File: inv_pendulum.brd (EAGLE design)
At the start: 55.5 x 77.5 mm, 9 parts

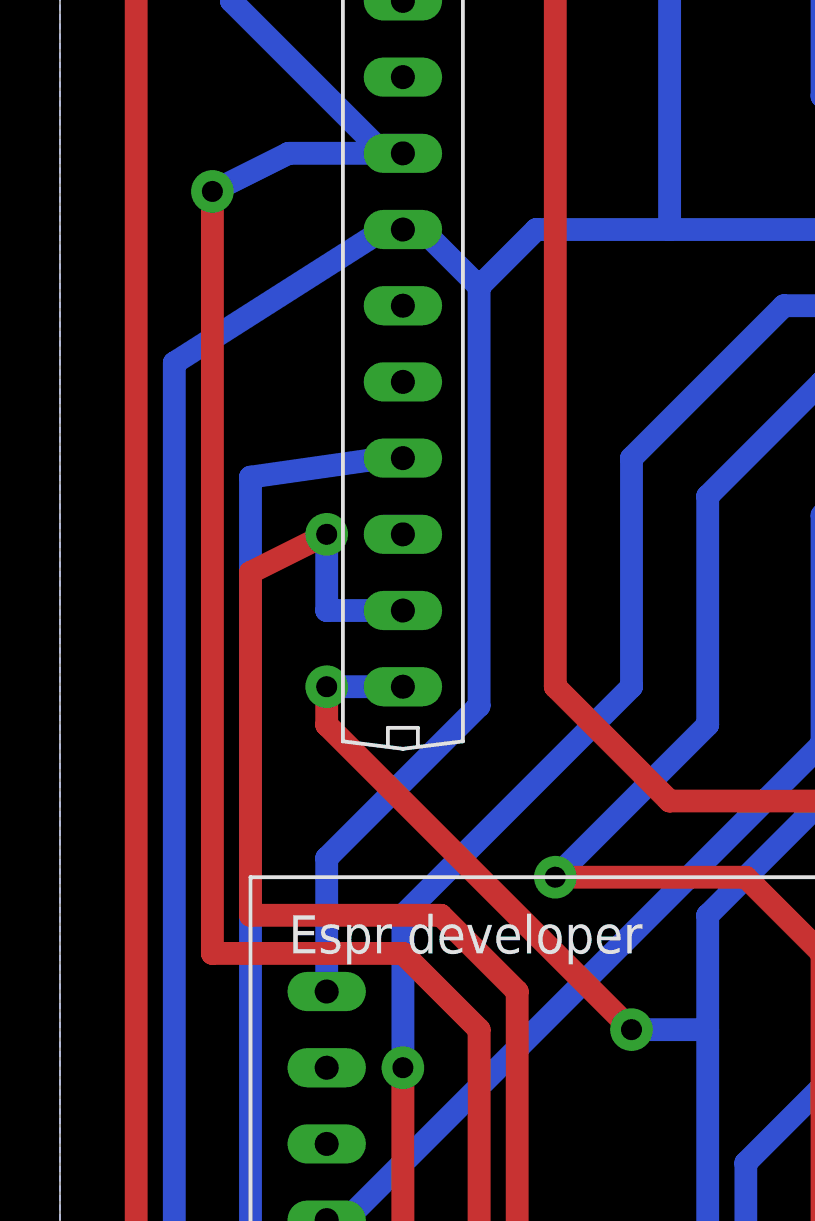
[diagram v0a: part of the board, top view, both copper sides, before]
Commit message: update design
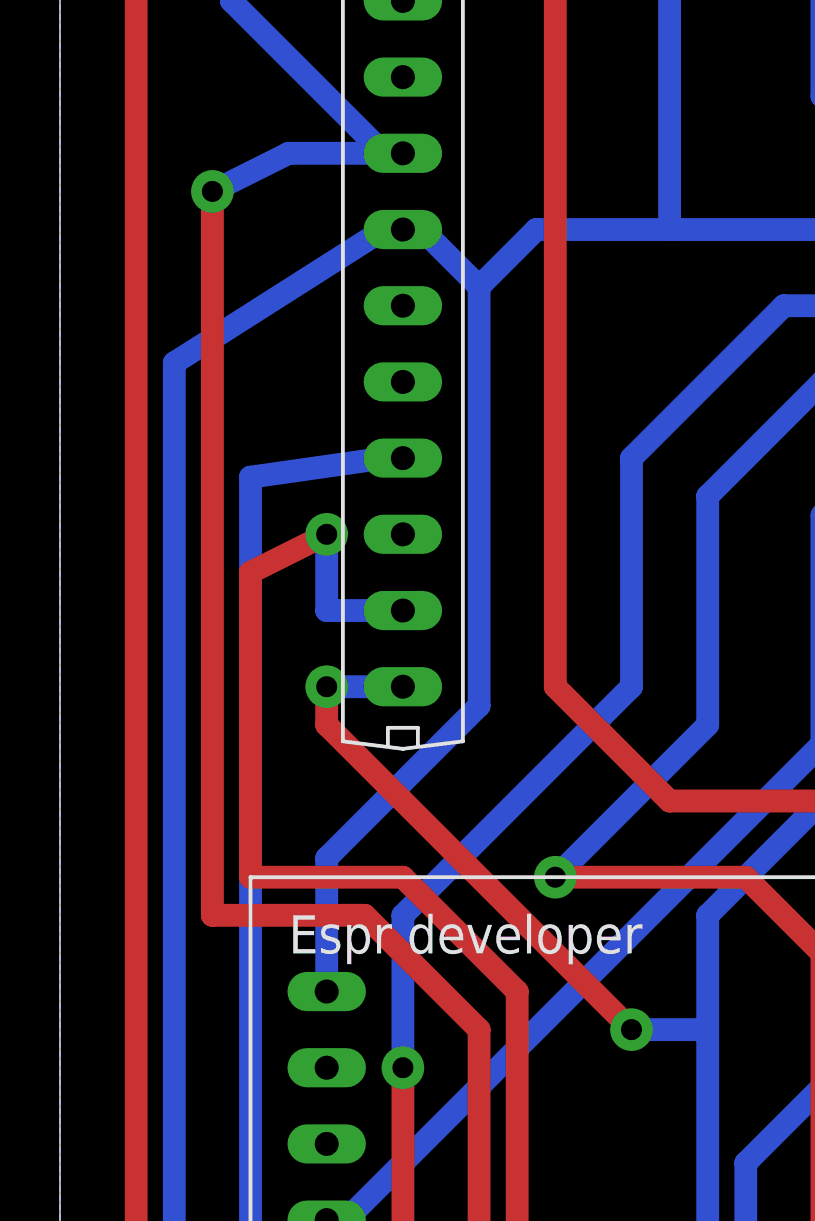
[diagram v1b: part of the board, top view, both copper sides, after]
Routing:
- net N$10: track 86.4 -> 85.6 mm
- net 6V: track 138.4 -> 137.6 mm
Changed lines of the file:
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@@
 <wire x1="16.51" y1="17.78" x2="13.97" y2="17.78" width="0.762" layer="1"/>
 <wire x1="13.97" y1="17.78" x2="13.97" y2="26.67" width="0.762" layer="1"/>
-<wire x1="13.97" y1="26.67" x2="11.43" y2="29.21" width="0.762" layer="1"/>
-<wire x1="11.43" y1="29.21" x2="5.08" y2="29.21" width="0.762" layer="1"/>
-<wire x1="5.08" y1="29.21" x2="5.08" y2="54.61" width="0.762" layer="1"/>
+<wire x1="13.97" y1="26.67" x2="10.16" y2="30.48" width="0.762" layer="1"/>
+<wire x1="10.16" y1="30.48" x2="5.08" y2="30.48" width="0.762" layer="1"/>
+<wire x1="5.08" y1="30.48" x2="5.08" y2="54.61" width="0.762" layer="1"/>
 <via x="5.08" y="54.61" extent="1-16" drill="0.7" diameter="1.4224"/>
 <wire x1="5.08" y1="54.61" x2="7.62" y2="55.88" width="0.762" layer="16"/>
@@
 <wire x1="19.05" y1="19.05" x2="15.24" y2="19.05" width="0.762" layer="1"/>
 <wire x1="15.24" y1="19.05" x2="15.24" y2="27.94" width="0.762" layer="1"/>
-<wire x1="15.24" y1="27.94" x2="12.7" y2="30.48" width="0.762" layer="1"/>
-<wire x1="12.7" y1="30.48" x2="6.35" y2="30.48" width="0.762" layer="1"/>
-<wire x1="6.35" y1="30.48" x2="6.35" y2="41.91" width="0.762" layer="1"/>
+<wire x1="15.24" y1="27.94" x2="11.43" y2="31.75" width="0.762" layer="1"/>
+<wire x1="11.43" y1="31.75" x2="6.35" y2="31.75" width="0.762" layer="1"/>
+<wire x1="6.35" y1="31.75" x2="6.35" y2="41.91" width="0.762" layer="1"/>
 <wire x1="6.35" y1="41.91" x2="8.89" y2="43.18" width="0.762" layer="1"/>
 <via x="8.89" y="43.18" extent="1-16" drill="0.7" diameter="1.4224"/>
